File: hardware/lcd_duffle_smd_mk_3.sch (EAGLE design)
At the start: 14 parts, among them IC1 ATTINY84, IC2 WS2811

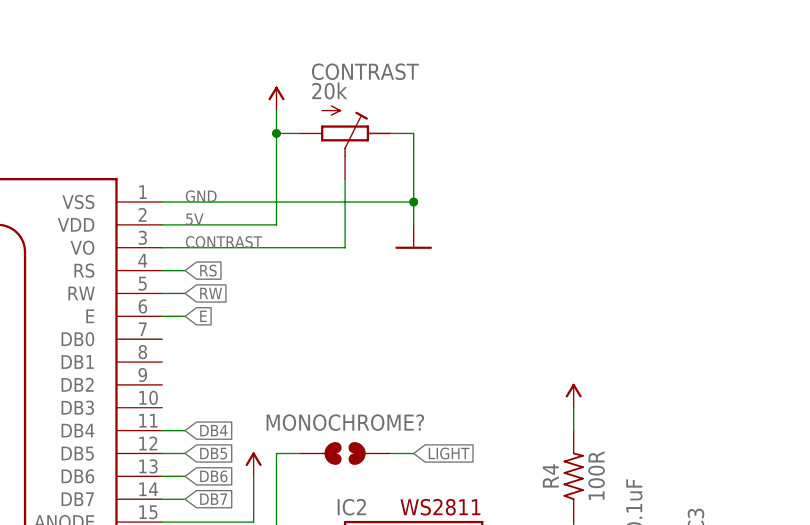
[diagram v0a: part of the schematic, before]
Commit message: ready for the fab
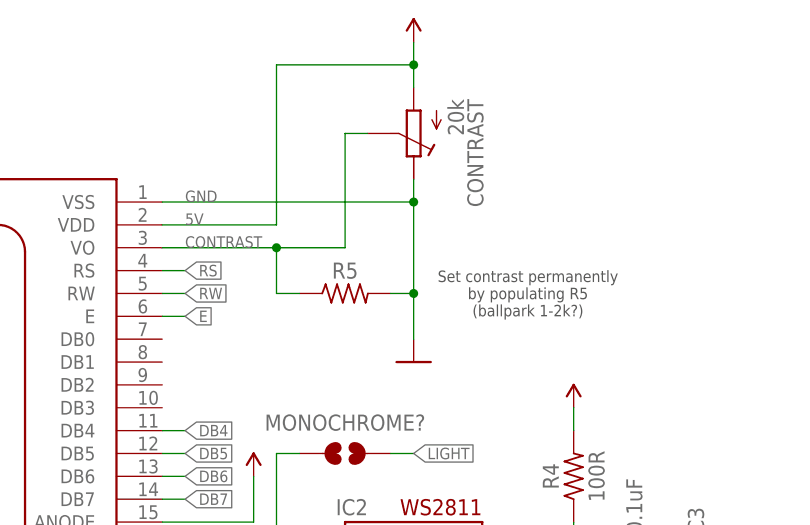
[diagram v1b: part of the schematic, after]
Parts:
- added R5: (no value), A_butts:RESISTORR0805
- CONTRAST: device A_butts:POTENTIOMETERTHUMBWHEEL-16MM -> A_butts:POTENTIOMETER3314Z
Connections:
- net CONTRAST: now also R5.1
- net GND: now also R5.2
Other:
- note added: "Set contrast permanently by populating R5 (ballpark 1-2k?)"
- moved on the sheet: CONTRAST
